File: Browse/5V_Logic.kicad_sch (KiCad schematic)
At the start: 9 parts, among them IC5 TPS2121RUXT

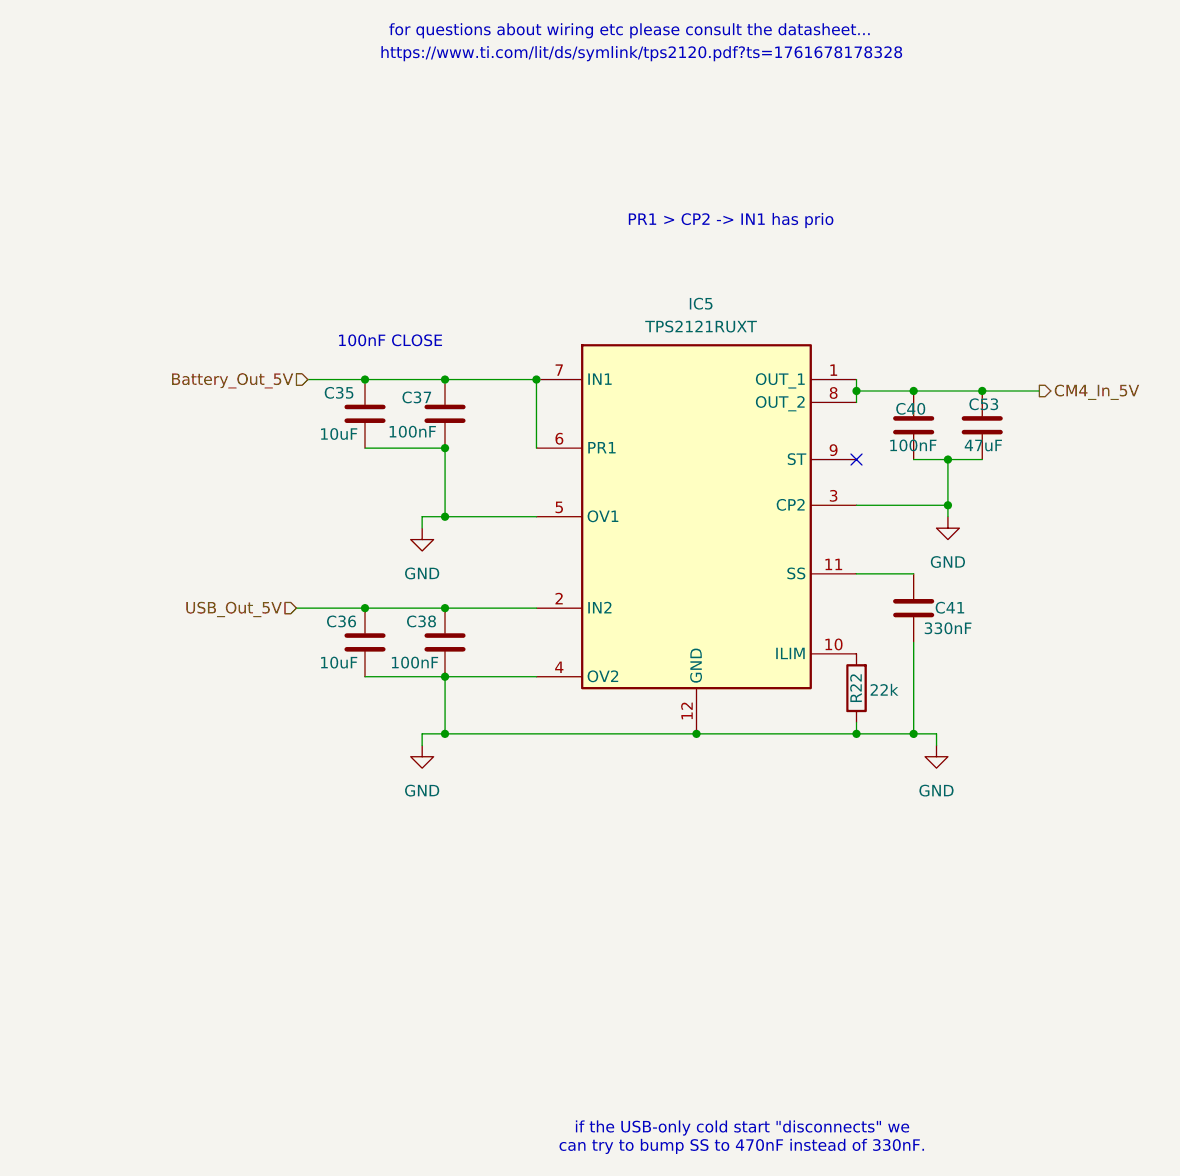
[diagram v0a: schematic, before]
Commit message: Deploying to gh-pages from @ Nautilus-UUV/nautilus-mainboard-PCB@5f5fdd9436d408a604bb268d740c0ac7ce1f5af5 🚀
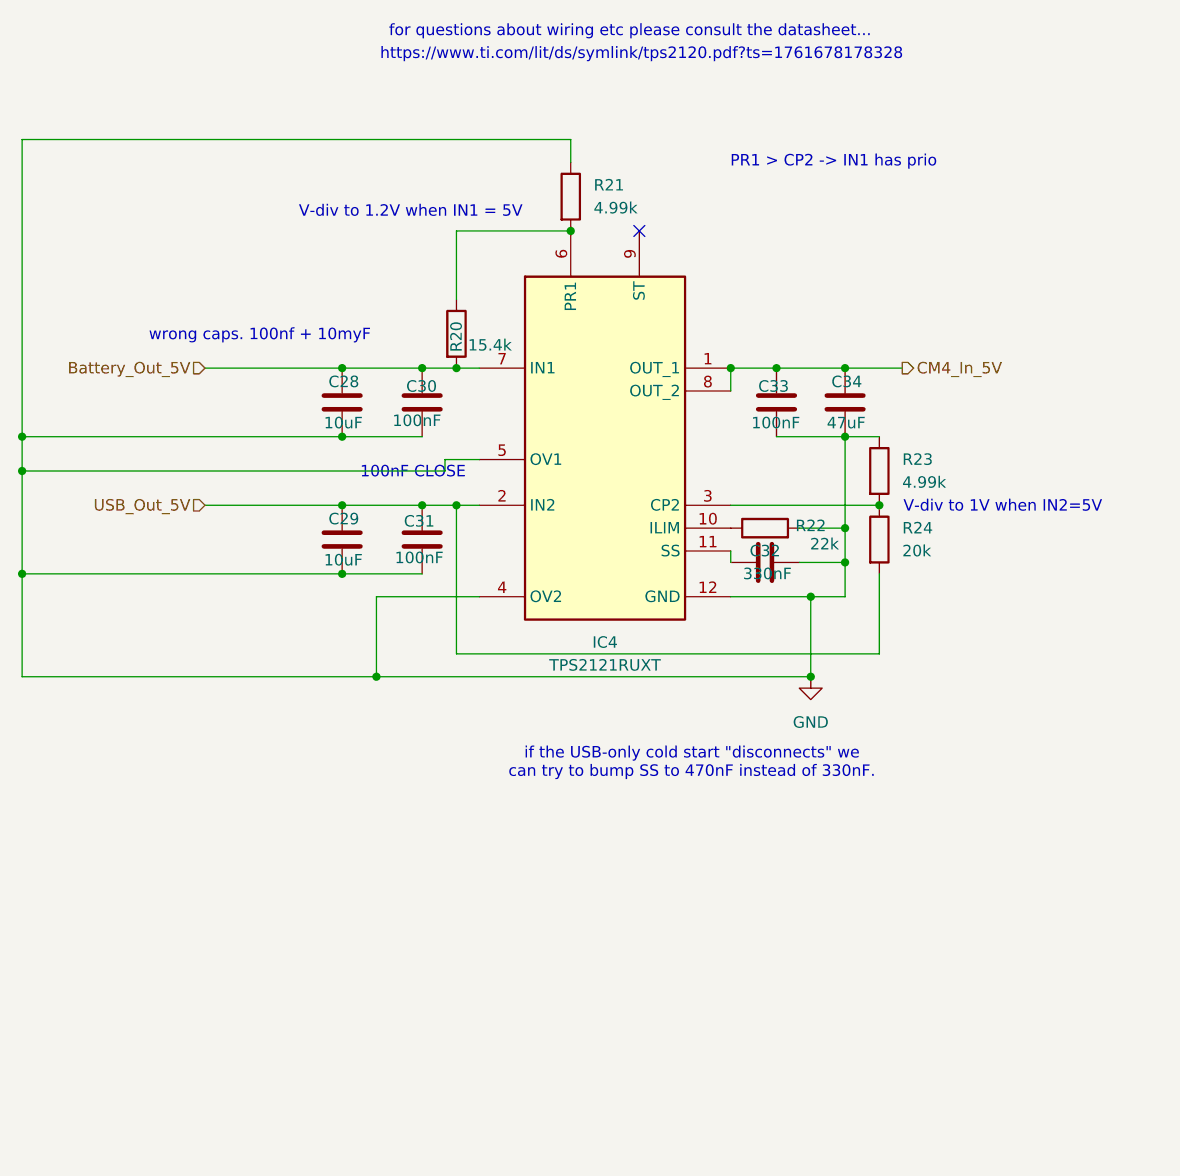
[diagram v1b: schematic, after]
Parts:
- removed C35, C36: 10uF, Capacitor_SMD:C_1210_3225Metric, symbol #dzdb:s_cap/C-MUR-GRM32EC72A106KE05
- removed C37, C38, C40: 100nF, Capacitor_SMD:C_0603_1608Metric, symbol #dzdb:g_cap/C-100n-0603
- removed C41: 330nF, Capacitor_SMD:C_0603_1608Metric, symbol #dzdb:g_cap/C-330n-0603
- removed C53: 47uF, Capacitor_SMD:C_0805_2012Metric, symbol #dzdb:s_cap/C-MUR-GRM21BR61A476ME15
- removed IC5: TPS2121RUXT, dz_dio:TI_Switchover_TPS2121RUXT, symbol #dzdb:s_misc/TEXA-595-TPS2121RUXT
- added C28, C29: 10uF, Capacitor_SMD:C_1210_3225Metric, symbol #dzdb:s_cap/C-MUR-GRM32EC72A106KE05
- added C30, C31, C33: 100nF, Capacitor_SMD:C_0603_1608Metric, symbol #dzdb:g_cap/C-100n-0603
- added C32: 330nF, Capacitor_SMD:C_0603_1608Metric, symbol #dzdb:g_cap/C-330n-0603
- added C34: 47uF, Capacitor_SMD:C_0805_2012Metric, symbol #dzdb:s_cap/C-MUR-GRM21BR61A476ME15
- added IC4: TPS2121RUXT, dz_dio:TI_Switchover_TPS2121RUXT, symbol #dzdb:s_misc/TEXA-595-TPS2121RUXT
- added R20: 15.4k, Resistor_SMD:R_0603_1608Metric, symbol #dzdb:g_res/R-15.4k-0603
- added R21, R23: 4.99k, Resistor_SMD:R_0603_1608Metric, symbol #dzdb:g_res/R-4.99k-0603
- added R24: 20k, Resistor_SMD:R_0603_1608Metric, symbol #dzdb:g_res/R-20k-0603
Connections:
- net Battery_Out_5V: now also C28.1, C30.1, IC4.7 (IN1), R20.2
- net CM4_In_5V: now also C33.1, C34.1, IC4.1 (OUT_1), IC4.8 (OUT_2)
- net GND: now also R22.2, C28.2, C29.2, C30.2, C31.2, C32.2, C33.2, C34.2, IC4.12 (GND), IC4.4 (OV2), IC4.5 (OV1), R21.1, R23.1; no longer R22.1
- net USB_Out_5V: now also C29.1, C31.1, IC4.2 (IN2), R24.2
- new net: IC4.3 (CP2), R23.2, R24.1
- new net: IC4.10 (ILIM), R22.1
- new net: IC4.6 (PR1), R20.1, R21.2
- new net: C32.1, IC4.11 (SS)
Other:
- note added: "V-div to 1.2V when IN1 = 5V"
- note added: "V-div to 1V when IN2=5V"
- note added: "wrong caps. 100nf + 10myF"
- company: Davide -> (none)
- title: Nautilus_Mainboard -> (none)
- moved on the sheet: R22

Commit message: Deploying to gh-pages from @ Nautilus-UUV/nautilus-mainboard-PCB@f1dd6ce1e57c066b805694b10777c719502cca87 🚀
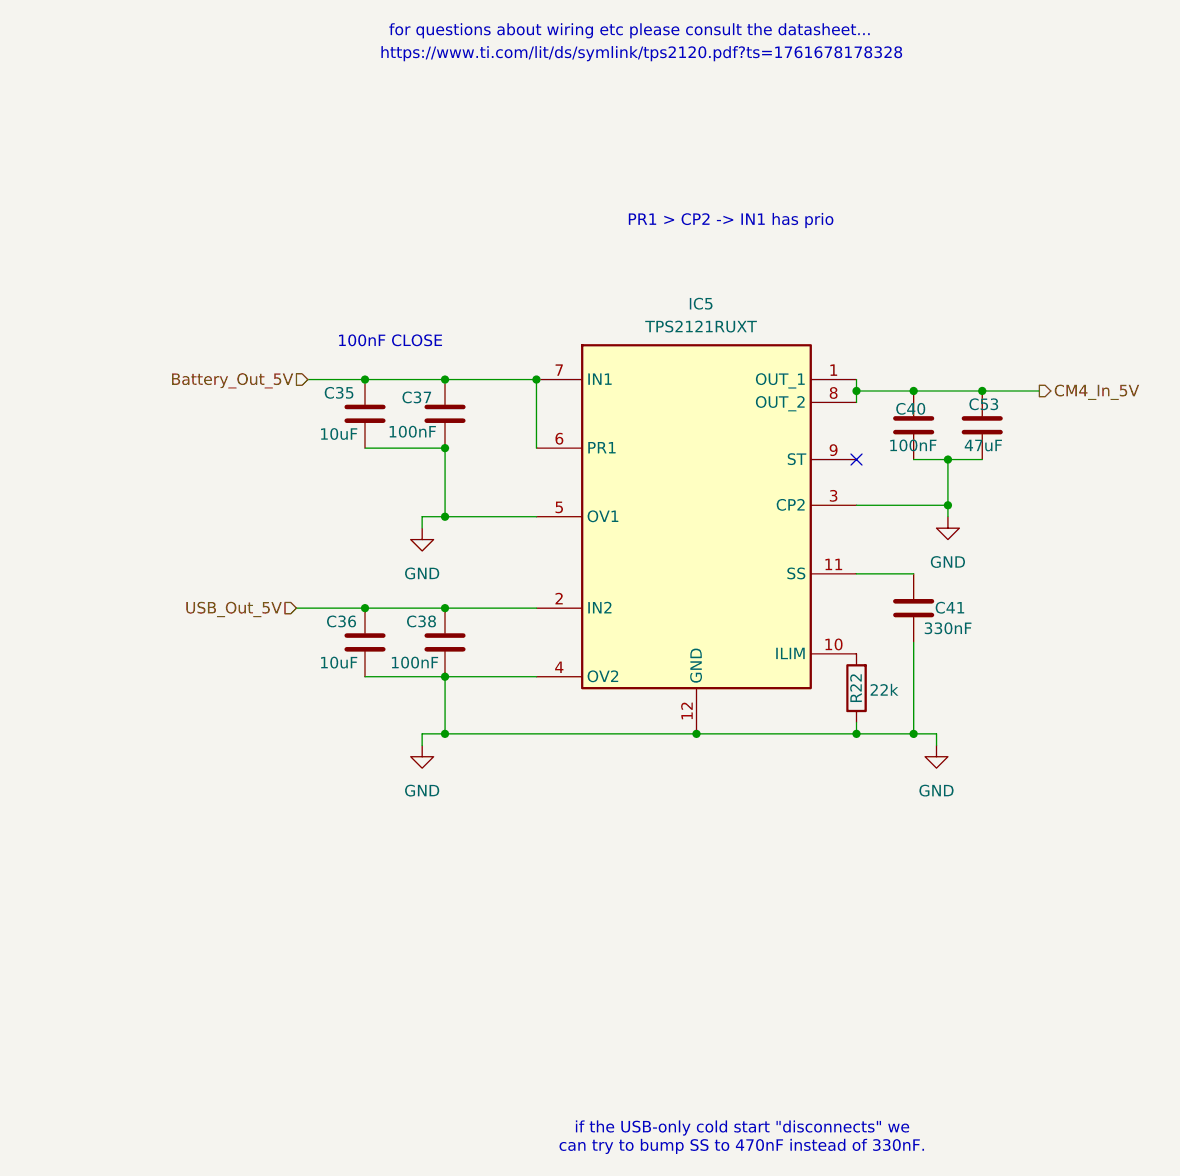
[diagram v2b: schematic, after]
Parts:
- removed C28, C29: 10uF, Capacitor_SMD:C_1210_3225Metric, symbol #dzdb:s_cap/C-MUR-GRM32EC72A106KE05
- removed C30, C31, C33: 100nF, Capacitor_SMD:C_0603_1608Metric, symbol #dzdb:g_cap/C-100n-0603
- removed C32: 330nF, Capacitor_SMD:C_0603_1608Metric, symbol #dzdb:g_cap/C-330n-0603
- removed C34: 47uF, Capacitor_SMD:C_0805_2012Metric, symbol #dzdb:s_cap/C-MUR-GRM21BR61A476ME15
- removed IC4: TPS2121RUXT, dz_dio:TI_Switchover_TPS2121RUXT, symbol #dzdb:s_misc/TEXA-595-TPS2121RUXT
- removed R20: 15.4k, Resistor_SMD:R_0603_1608Metric, symbol #dzdb:g_res/R-15.4k-0603
- removed R21, R23: 4.99k, Resistor_SMD:R_0603_1608Metric, symbol #dzdb:g_res/R-4.99k-0603
- removed R24: 20k, Resistor_SMD:R_0603_1608Metric, symbol #dzdb:g_res/R-20k-0603
- added C35, C36: 10uF, Capacitor_SMD:C_1210_3225Metric, symbol #dzdb:s_cap/C-MUR-GRM32EC72A106KE05
- added C37, C38, C40: 100nF, Capacitor_SMD:C_0603_1608Metric, symbol #dzdb:g_cap/C-100n-0603
- added C41: 330nF, Capacitor_SMD:C_0603_1608Metric, symbol #dzdb:g_cap/C-330n-0603
- added C53: 47uF, Capacitor_SMD:C_0805_2012Metric, symbol #dzdb:s_cap/C-MUR-GRM21BR61A476ME15
- added IC5: TPS2121RUXT, dz_dio:TI_Switchover_TPS2121RUXT, symbol #dzdb:s_misc/TEXA-595-TPS2121RUXT
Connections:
- net Battery_Out_5V: now also C35.1, C37.1, IC5.6 (PR1), IC5.7 (IN1)
- net CM4_In_5V: now also C40.1, C53.1, IC5.1 (OUT_1), IC5.8 (OUT_2)
- net GND: now also R22.1, C35.2, C36.2, C37.2, C38.2, C40.2, C41.1, C53.2, IC5.12 (GND), IC5.3 (CP2), IC5.4 (OV2), IC5.5 (OV1); no longer R22.2
- net USB_Out_5V: now also C36.1, C38.1, IC5.2 (IN2)
- new net: C41.2, IC5.11 (SS)
- new net: IC5.10 (ILIM), R22.2
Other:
- note removed: "V-div to 1.2V when IN1 = 5V"
- note removed: "V-div to 1V when IN2=5V"
- note removed: "wrong caps. 100nf + 10myF"
- company: (none) -> Davide
- title: (none) -> Nautilus_Mainboard
- moved on the sheet: R22
